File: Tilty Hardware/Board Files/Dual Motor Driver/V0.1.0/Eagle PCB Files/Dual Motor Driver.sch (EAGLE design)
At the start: 25 parts, among them U1 ATMEGA32U4TQFP, U2 L298_BRIDGE_DRIVER

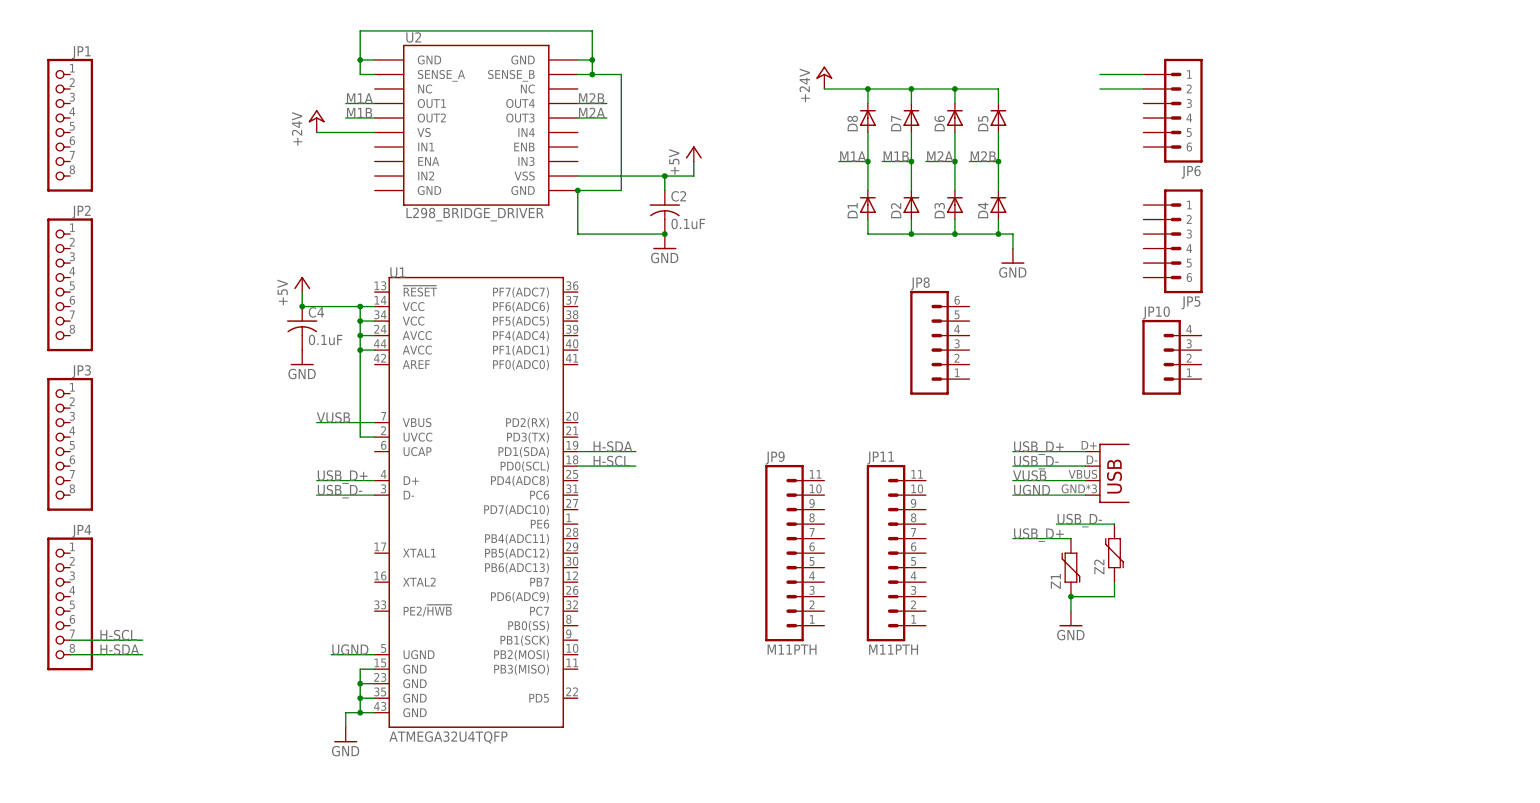
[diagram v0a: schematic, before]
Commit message: Lots of work on dual motor driver
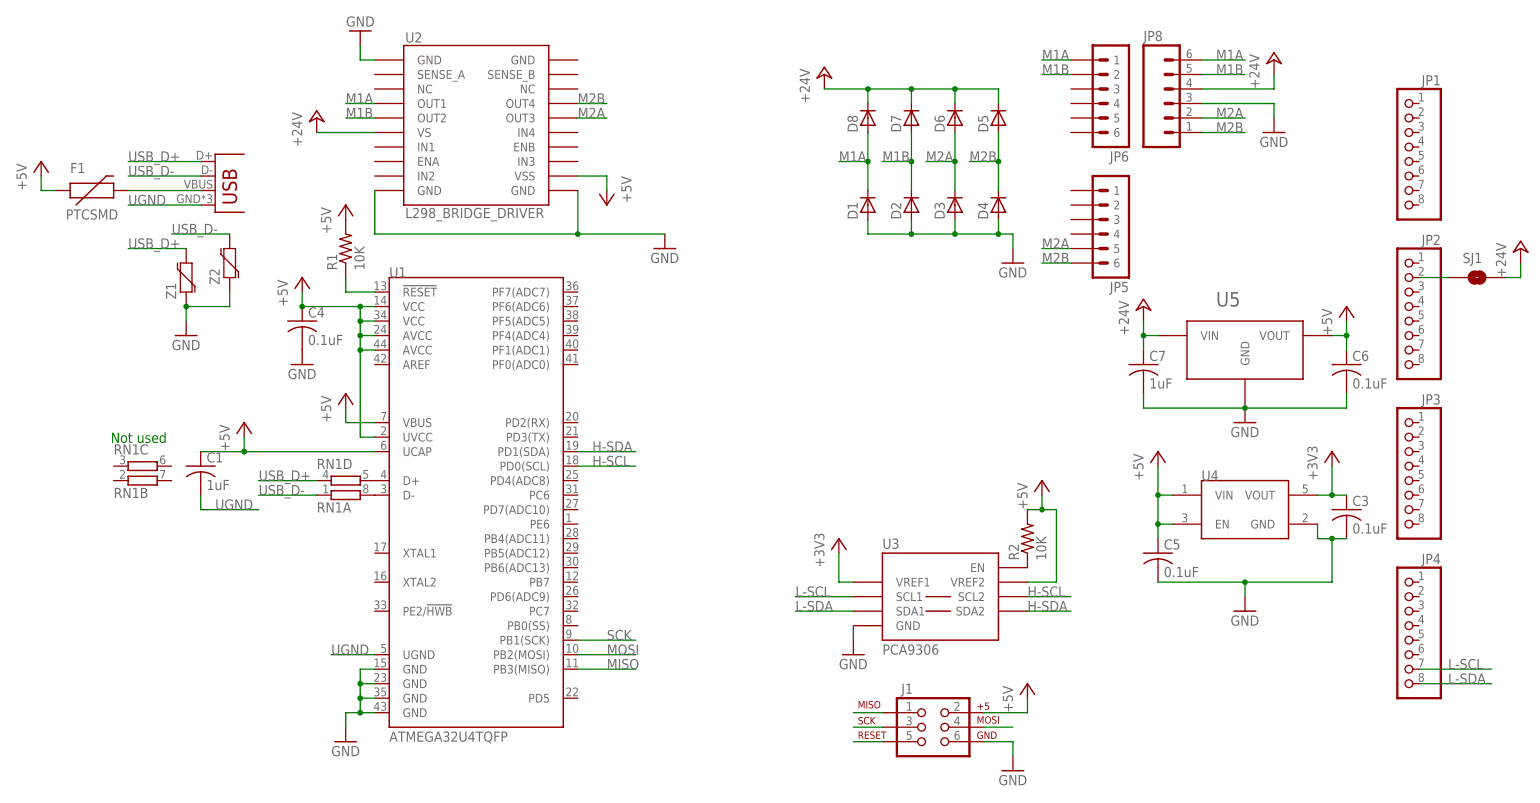
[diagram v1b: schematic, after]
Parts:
- removed C2: 0.1uF, resistor:C-USC0603
- removed JP10: (no value), SparkFun-Connectors:M04SMD2
- removed JP11, JP9: M11PTH, SparkFun-Connectors:M11PTH
- added C1, C7: 1uF, resistor:C-USC0603
- added C3, C5, C6: 0.1uF, resistor:C-USC0603
- added F1: PTCSMD, SparkFun-PowerIC:PTCSMD
- added J1: AVR_SPI_PRG_6PTH, SparkFun-Connectors:AVR_SPI_PRG_6PTH
- added R1, R2: 10K, resistor:R-US_R0603
- added RN1: (no value), resistor-dil:4R-N0603-ARV
- added SJ1: SOLDERJUMPERNC, SparkFun-Passives:SOLDERJUMPERNC
- added U3: PCA9306, My Parts:PCA9306
- added U4: TLV71333PDBVR, SparkFun-PowerIC:ADP160
- added U5: VOLTAGE-REGULATOR, My Parts:VOLTAGE-REGULATOR
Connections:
- removed net VUSB: JP7.VBUS, U1.VBUS
- new net +3V3: C3.1, U3.VREF1, U4.VOUT
- new net L-SCL: JP4.7, U3.SCL1
- new net L-SDA: JP4.8, U3.SDA1
- new net MISO: J1.1, U1.PB3(MISO)
- new net MOSI: J1.4, U1.PB2(MOSI)
- new net N$1: RN1D.2, U1.D+
- new net N$2: RN1A.2, U1.D-
- new net N$3: R2.1, U3.EN
- new net N$4: F1.2, JP7.VBUS
- new net N$5: JP2.2, SJ1.1
- new net RESET: J1.5, R1.1, U1.!RESET
- new net SCK: J1.3, U1.PB1(SCK)
- net +24V: now also C7.1, JP8.4, SJ1.2, U5.VIN
- net +5V: now also C1.1, C5.1, C6.1, F1.1, J1.2, R1.2, R2.2, U1.UCAP, U1.VBUS, U3.VREF2, U4.EN, U4.VIN, U5.VOUT; no longer C2.1
- net GND: now also C3.2, C5.2, C6.2, C7.2, J1.6, JP8.3, U2.GND@10, U3.GND, U4.GND, U5.GND; no longer C2.2, U2.GND@20, U2.SENSE_A, U2.SENSE_B
- net H-SCL: now also U3.SCL2; no longer JP4.7
- net H-SDA: now also U3.SDA2; no longer JP4.8
- net M1A: now also JP8.6
- net M1B: now also JP8.5
- net M2A: now also JP5.5, JP8.2
- net M2B: now also JP5.6, JP8.1
- net UGND: now also C1.2
- net USB_D+: now also RN1D.1; no longer U1.D+
- net USB_D-: now also RN1A.1; no longer U1.D-
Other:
- note added: "Not used"
- moved on the sheet: JP1, JP2, JP3, JP4, JP5, JP6, JP8, Z1, Z2
